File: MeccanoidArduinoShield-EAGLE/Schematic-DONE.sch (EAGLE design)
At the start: 31 parts

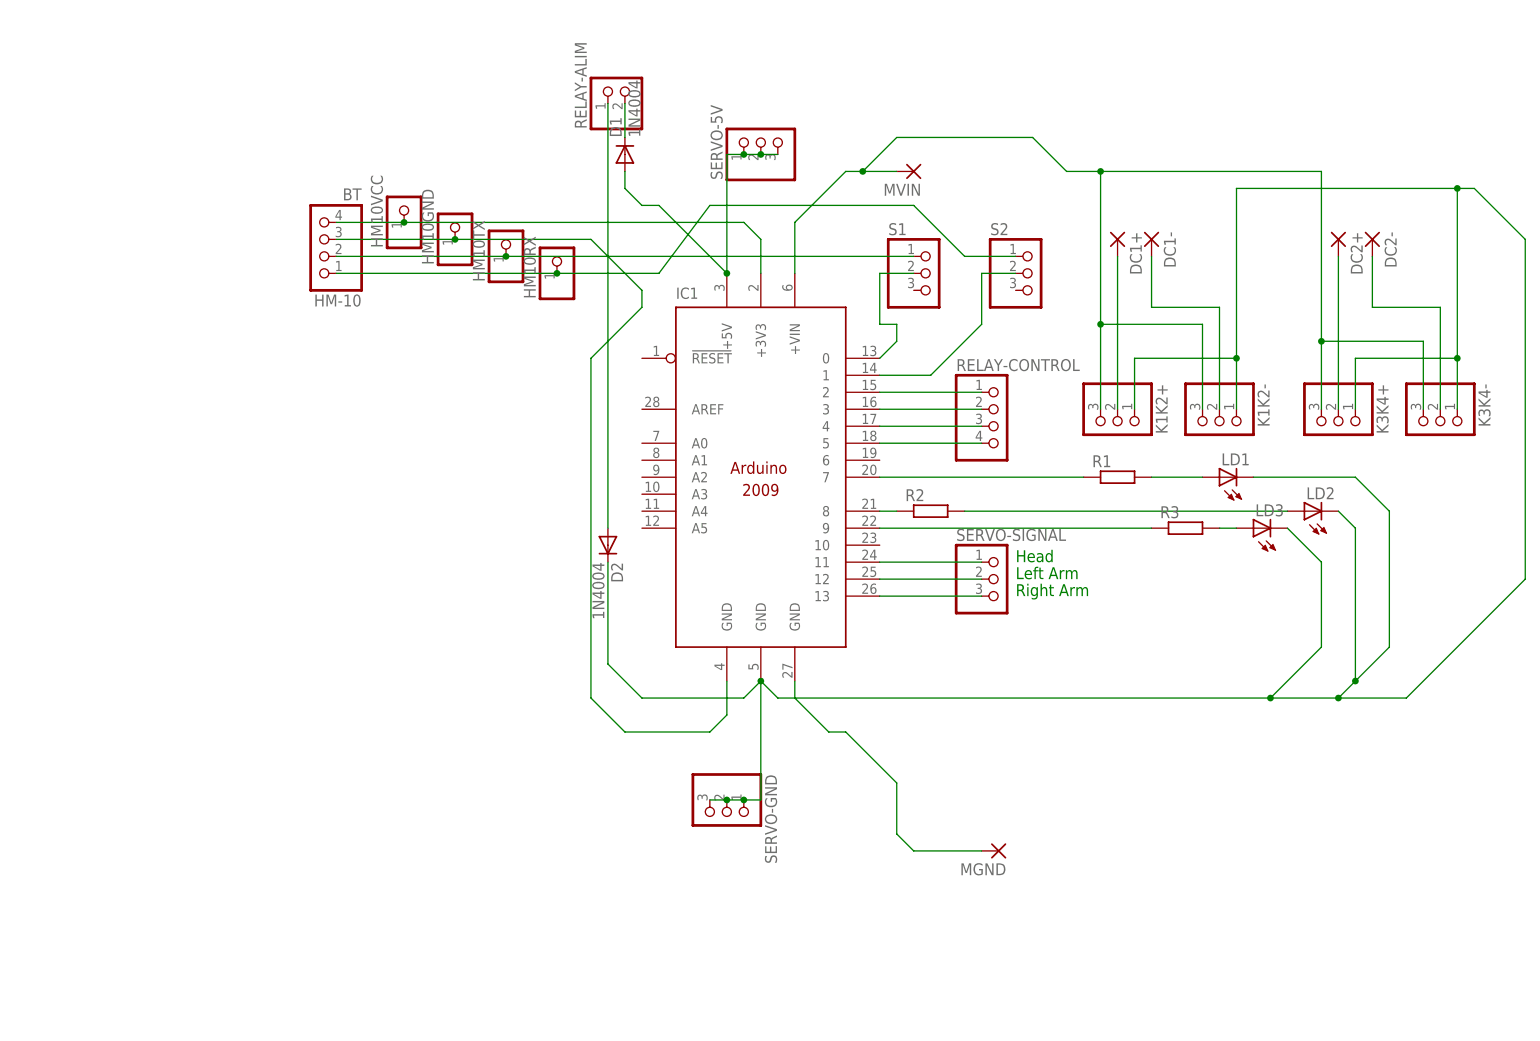
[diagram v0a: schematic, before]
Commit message: Update content for youtube video
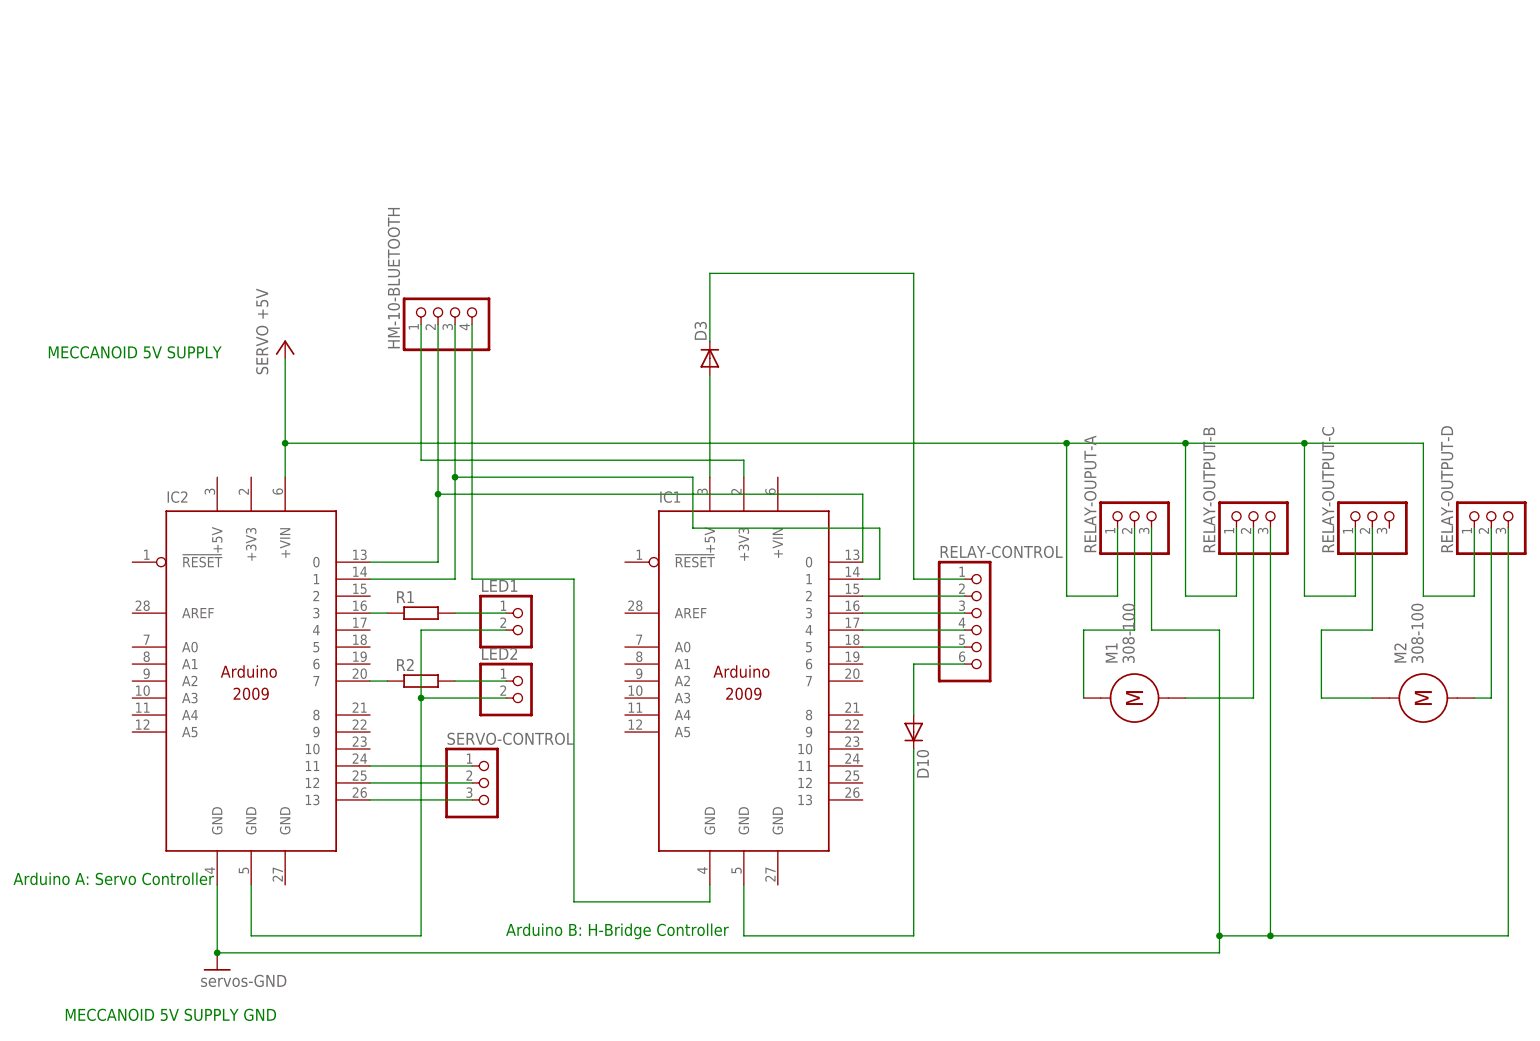
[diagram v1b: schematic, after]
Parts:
- removed D1, D2: 1N4004, diode:1N4004
- removed DC1+, DC1-, DC2+, DC2-, MGND, MVIN: (no value), wirepad:3,17/1,3
- removed HM-10: BT, pinhead:PINHD-1X4
- removed HM10GND, HM10RX, HM10TX, HM10VCC: (no value), pinhead:PINHD-1X1
- removed K1K2+, K1K2-, K3K4+, K3K4-: (no value), pinhead:PINHD-1X3/90
- removed LD1, LD2, LD3: (no value), led:LED3MM
- removed R3: (no value), resistor:R-EU_0207/10
- removed RELAY-ALIM: (no value), pinhead:PINHD-1X2
- removed S1, S2, SERVO-5V, SERVO-GND, SERVO-SIGNAL: (no value), pinhead:PINHD-1X3
- added D10, D3: 1N4148DO35-7, diode:1N4148DO35-7
- added HM-10-BLUETOOTH: (no value), pinhead:PINHD-1X4
- added IC2: (no value), arduino:ARDUINO2009_10
- added LED1, LED2: (no value), pinhead:PINHD-1X2
- added M1, M2: 308-100, motor:308-100
- added RELAY-OUPUT-A, RELAY-OUTPUT-B, RELAY-OUTPUT-C, RELAY-OUTPUT-D, SERVO-CONTROL: (no value), pinhead:PINHD-1X3
- IC1: OC_FARNELL unknown -> (none)
- R1, R2: device resistor:R-EU_0207/10 -> resistor:R-EU_0204/2V
- RELAY-CONTROL: device pinhead:PINHD-1X4 -> pinhead:PINHD-1X6; OC_FARNELL unknown -> (none)
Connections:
- removed net N$14: IC1.4, RELAY-CONTROL.3
- removed net N$25: LD3.A, R3.2
- removed net N$26: IC1.9, R3.1
- removed net N$27: IC1.8, R2.1
- removed net N$28: DC2+.P, K3K4+.2
- removed net N$31: D2.C, IC1.GND@2, K1K2+.1, K1K2-.1, K3K4+.1, K3K4-.1, LD1.C, LD2.C, LD3.C, SERVO-GND.1, SERVO-GND.2, SERVO-GND.3
- removed net N$32: IC1.+VIN, K1K2+.3, K1K2-.3, K3K4+.3, K3K4-.3, MVIN.P
- new net +5V: IC2.+VIN, RELAY-OUPUT-A.1, RELAY-OUTPUT-B.1, RELAY-OUTPUT-C.1, RELAY-OUTPUT-D.1
- new net GND: IC2.GND@1, RELAY-OUPUT-A.3, RELAY-OUTPUT-B.3, RELAY-OUTPUT-D.3
- new net N$23: LED2.1, R2.2
- new net RELAY-OUTPUT-D: M2.NEG, RELAY-OUTPUT-D.2
- net N$1: now also M1.POS, RELAY-OUPUT-A.2; no longer HM-10.3, HM10GND.1, IC1.GND@1
- net N$10: now also M1.NEG, RELAY-OUTPUT-B.2; no longer IC1.12, SERVO-SIGNAL.2
- net N$11: now also IC2.11, SERVO-CONTROL.1; no longer IC1.11, SERVO-SIGNAL.1
- net N$12: now also D10.C, IC1.GND@2; no longer IC1.2, RELAY-CONTROL.1
- net N$13: now also IC2.12, SERVO-CONTROL.2; no longer IC1.3, RELAY-CONTROL.2
- net N$15: now also IC2.13, SERVO-CONTROL.3; no longer IC1.5, RELAY-CONTROL.4
- net N$16: now also HM-10-BLUETOOTH.1, IC1.+3V3; no longer D2.A, RELAY-ALIM.1
- net N$17: now also D10.A, RELAY-CONTROL.6; no longer IC1.7, R1.1
- net N$18: now also HM-10-BLUETOOTH.2, IC1.0, IC2.0; no longer DC1+.P, K1K2+.2
- net N$19: now also HM-10-BLUETOOTH.4, IC1.GND@1; no longer IC1.1, S2.2
- net N$2: now also M2.POS, RELAY-OUTPUT-C.2; no longer HM-10.4, HM10VCC.1, IC1.+3V3
- net N$20: now also HM-10-BLUETOOTH.3, IC1.1, IC2.1; no longer HM-10.1, HM10RX.1, S2.1
- net N$21: now also LED1.1; no longer LD1.A
- net N$22: now also IC2.GND@2, LED1.2, LED2.2; no longer DC2-.P, K3K4-.2
- net N$24: now also IC2.7, R2.1; no longer LD2.A, R2.2
- net N$3: now also D3.C, RELAY-CONTROL.1; no longer IC1.0, S1.2
- net N$4: now also IC1.2, RELAY-CONTROL.2; no longer D1.A, IC1.+5V, SERVO-5V.1, SERVO-5V.2, SERVO-5V.3
- net N$5: now also IC1.3, RELAY-CONTROL.3; no longer HM-10.2, HM10TX.1, S1.1
- net N$6: now also IC1.4, RELAY-CONTROL.4; no longer D1.C, RELAY-ALIM.2
- net N$7: now also IC1.5, RELAY-CONTROL.5; no longer IC1.GND@3, MGND.P
- net N$8: now also D3.A, IC1.+5V; no longer DC1-.P, K1K2-.2
- net N$9: now also IC2.3, R1.1; no longer IC1.13, SERVO-SIGNAL.3
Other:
- note added: "Arduino A: Servo Controller"
- note added: "Arduino B: H-Bridge Controller"
- note added: "MECCANOID 5V SUPPLY"
- note added: "MECCANOID 5V SUPPLY GND"
- note removed: "Head"
- note removed: "Left Arm"
- note removed: "Right Arm"
- moved on the sheet: IC1, R1, R2
